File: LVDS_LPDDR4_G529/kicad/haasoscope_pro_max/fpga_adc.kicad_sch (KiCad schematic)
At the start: 0 parts

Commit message: Aligned schematics, sort of
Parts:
- added IC1: ADC12DL500ACF_Aligned, ADC12DL:BGA256C100P16X16_1700X1700X331, symbol Aligned_Peripheral_Symbols:ADC12DL500ACF_Aligned
- added U3: Ti90G529_Functions, G529:BGA-529_23x23_19.0x19.0mm, symbol Ti90G529_Functions:Ti90G529_Functions

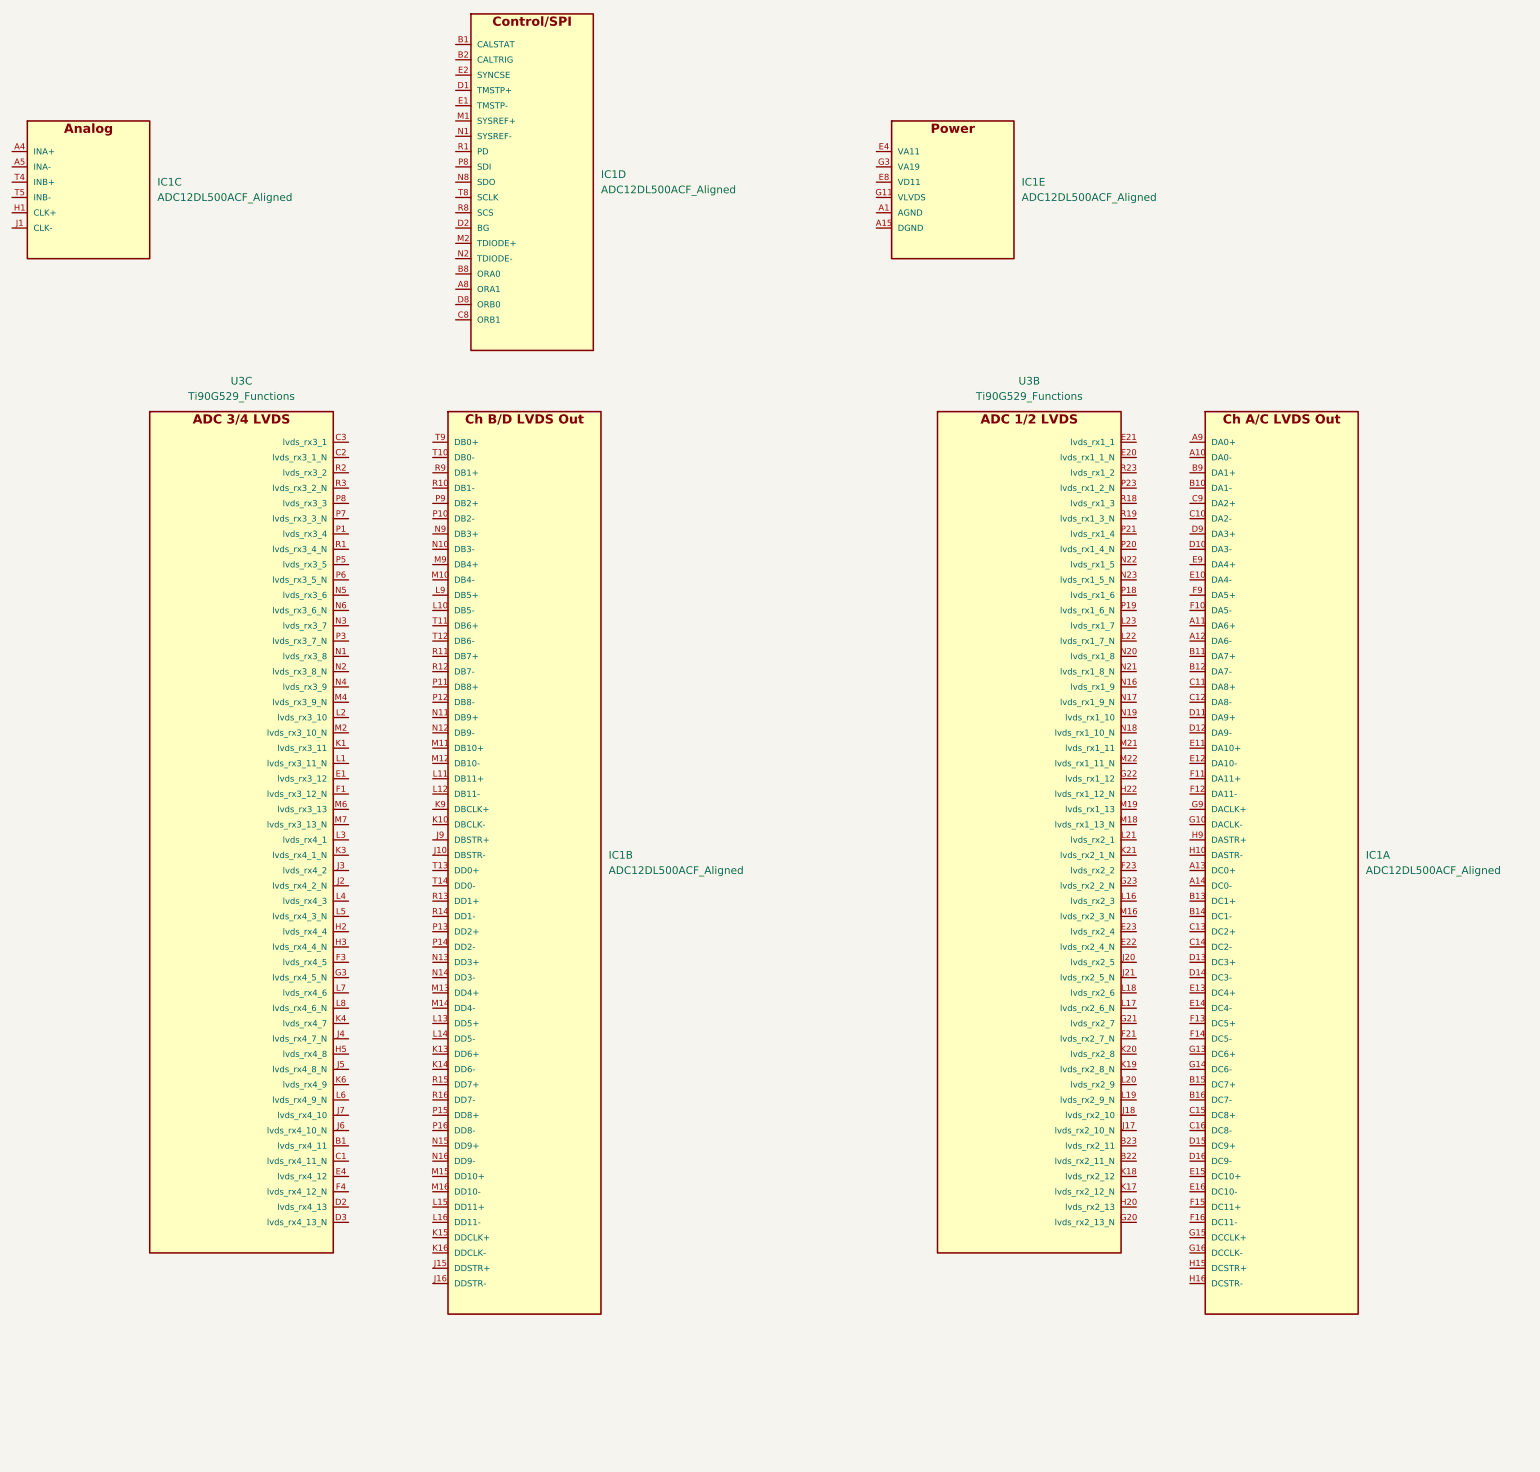
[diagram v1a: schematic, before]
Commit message: Aligned schematics, sort of
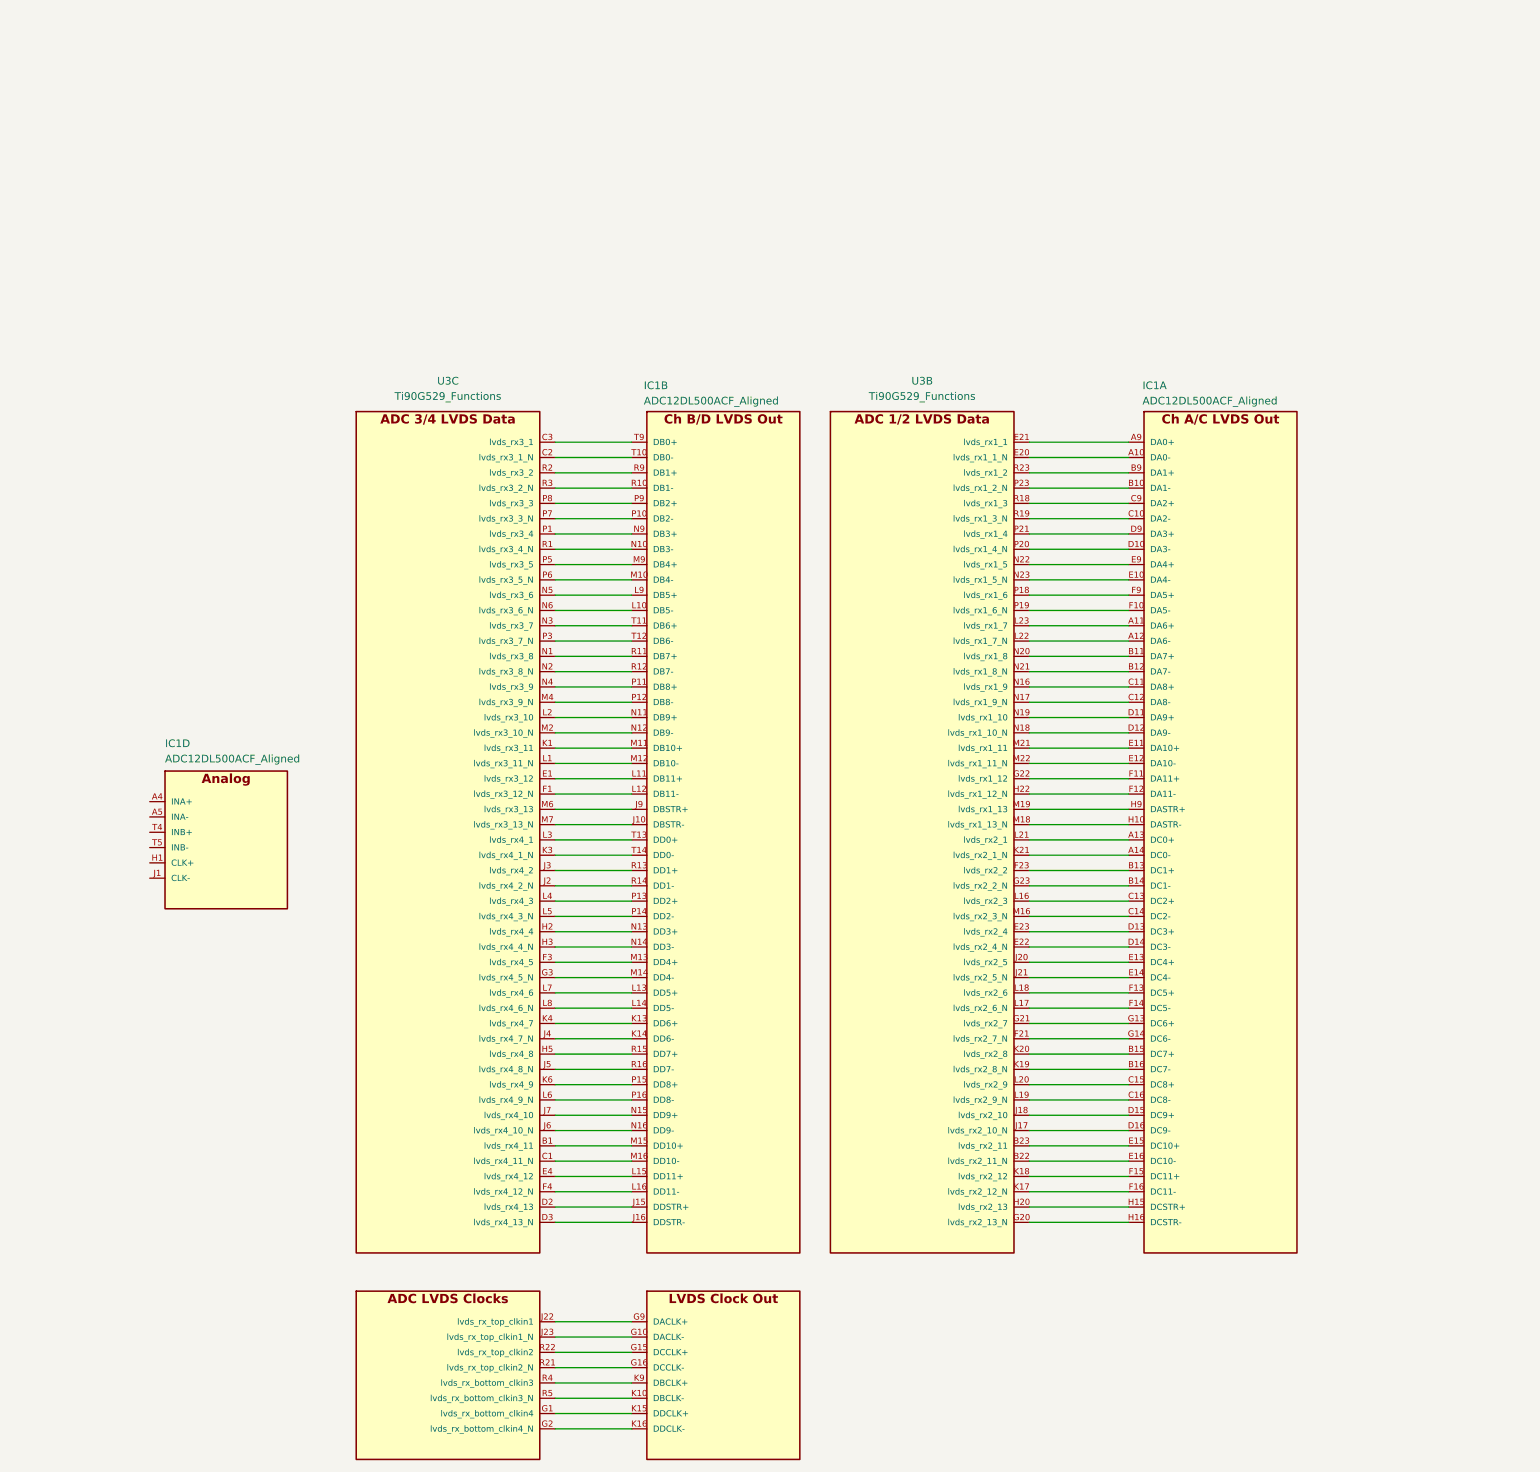
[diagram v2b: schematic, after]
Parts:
- removed unit 5 of IC1
- added unit 4 of U3
- IC1: footprint ADC12DL:BGA256C100P16X16_1700X1700X331 -> BGA256C100P16X16_1700X1700X331
- U3: footprint G529:BGA-529_23x23_19.0x19.0mm -> haasoscope_pro_adc_fpga_board:BGA-529_23x23_19.0x19.0mm
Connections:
- net at U3.B1 (lvds_rx4_11): now also IC1.M15 (DD10+)
- net at U3.C1 (lvds_rx4_11_N): now also IC1.M16 (DD10-)
- net at U3.C2 (lvds_rx3_1_N): now also IC1.T10 (DB0-)
- net at U3.C3 (lvds_rx3_1): now also IC1.T9 (DB0+)
- net at U3.D2 (lvds_rx4_13): now also IC1.J15 (DDSTR+)
- net at U3.D3 (lvds_rx4_13_N): now also IC1.J16 (DDSTR-)
- net at U3.E1 (lvds_rx3_12): now also IC1.L11 (DB11+)
- net at U3.E4 (lvds_rx4_12): now also IC1.L15 (DD11+)
- net at U3.F1 (lvds_rx3_12_N): now also IC1.L12 (DB11-)
- net at U3.F3 (lvds_rx4_5): now also IC1.M13 (DD4+)
- net at U3.F4 (lvds_rx4_12_N): now also IC1.L16 (DD11-)
- net at U3.G3 (lvds_rx4_5_N): now also IC1.M14 (DD4-)
- net at U3.H2 (lvds_rx4_4): now also IC1.N13 (DD3+)
- net at U3.H3 (lvds_rx4_4_N): now also IC1.N14 (DD3-)
- net at U3.H5 (lvds_rx4_8): now also IC1.R15 (DD7+)
- net at U3.J2 (lvds_rx4_2_N): now also IC1.R14 (DD1-)
- net at U3.J3 (lvds_rx4_2): now also IC1.R13 (DD1+)
- net at U3.J4 (lvds_rx4_7_N): now also IC1.K14 (DD6-)
- net at U3.J5 (lvds_rx4_8_N): now also IC1.R16 (DD7-)
- net at U3.J6 (lvds_rx4_10_N): now also IC1.N16 (DD9-)
- net at U3.J7 (lvds_rx4_10): now also IC1.N15 (DD9+)
- net at U3.K1 (lvds_rx3_11): now also IC1.M11 (DB10+)
- net at U3.K3 (lvds_rx4_1_N): now also IC1.T14 (DD0-)
- net at U3.K4 (lvds_rx4_7): now also IC1.K13 (DD6+)
- net at U3.K6 (lvds_rx4_9): now also IC1.P15 (DD8+)
- net at U3.L1 (lvds_rx3_11_N): now also IC1.M12 (DB10-)
- net at U3.L2 (lvds_rx3_10): now also IC1.N11 (DB9+)
- net at U3.L3 (lvds_rx4_1): now also IC1.T13 (DD0+)
- net at U3.L4 (lvds_rx4_3): now also IC1.P13 (DD2+)
- net at U3.L5 (lvds_rx4_3_N): now also IC1.P14 (DD2-)
- net at U3.L6 (lvds_rx4_9_N): now also IC1.P16 (DD8-)
- net at U3.L7 (lvds_rx4_6): now also IC1.L13 (DD5+)
- net at U3.L8 (lvds_rx4_6_N): now also IC1.L14 (DD5-)
- net at U3.M2 (lvds_rx3_10_N): now also IC1.N12 (DB9-)
- net at U3.M4 (lvds_rx3_9_N): now also IC1.P12 (DB8-)
- net at U3.M6 (lvds_rx3_13): now also IC1.J9 (DBSTR+)
- net at U3.M7 (lvds_rx3_13_N): now also IC1.J10 (DBSTR-)
- net at U3.N1 (lvds_rx3_8): now also IC1.R11 (DB7+)
- net at U3.N2 (lvds_rx3_8_N): now also IC1.R12 (DB7-)
- net at U3.N3 (lvds_rx3_7): now also IC1.T11 (DB6+)
- net at U3.N4 (lvds_rx3_9): now also IC1.P11 (DB8+)
- net at U3.N5 (lvds_rx3_6): now also IC1.L9 (DB5+)
- net at U3.N6 (lvds_rx3_6_N): now also IC1.L10 (DB5-)
- net at U3.P1 (lvds_rx3_4): now also IC1.N9 (DB3+)
- net at U3.P3 (lvds_rx3_7_N): now also IC1.T12 (DB6-)
- net at U3.P5 (lvds_rx3_5): now also IC1.M9 (DB4+)
- net at U3.P6 (lvds_rx3_5_N): now also IC1.M10 (DB4-)
- net at U3.P7 (lvds_rx3_3_N): now also IC1.P10 (DB2-)
- net at U3.P8 (lvds_rx3_3): now also IC1.P9 (DB2+)
- net at U3.R1 (lvds_rx3_4_N): now also IC1.N10 (DB3-)
- net at U3.R2 (lvds_rx3_2): now also IC1.R9 (DB1+)
- net at U3.R3 (lvds_rx3_2_N): now also IC1.R10 (DB1-)
- net at U3.B22 (lvds_rx2_11_N): now also IC1.E16 (DC10-)
- net at U3.B23 (lvds_rx2_11): now also IC1.E15 (DC10+)
- net at U3.E20 (lvds_rx1_1_N): now also IC1.A10 (DA0-)
- net at U3.E21 (lvds_rx1_1): now also IC1.A9 (DA0+)
- net at U3.E22 (lvds_rx2_4_N): now also IC1.D14 (DC3-)
- net at U3.E23 (lvds_rx2_4): now also IC1.D13 (DC3+)
- net at U3.F21 (lvds_rx2_7_N): now also IC1.G14 (DC6-)
- net at U3.F23 (lvds_rx2_2): now also IC1.B13 (DC1+)
- net at U3.G20 (lvds_rx2_13_N): now also IC1.H16 (DCSTR-)
- net at U3.G21 (lvds_rx2_7): now also IC1.G13 (DC6+)
- net at U3.G22 (lvds_rx1_12): now also IC1.F11 (DA11+)
- net at U3.G23 (lvds_rx2_2_N): now also IC1.B14 (DC1-)
- net at U3.H20 (lvds_rx2_13): now also IC1.H15 (DCSTR+)
- net at U3.H22 (lvds_rx1_12_N): now also IC1.F12 (DA11-)
- net at U3.J17 (lvds_rx2_10_N): now also IC1.D16 (DC9-)
- net at U3.J18 (lvds_rx2_10): now also IC1.D15 (DC9+)
- net at U3.J20 (lvds_rx2_5): now also IC1.E13 (DC4+)
- net at U3.J21 (lvds_rx2_5_N): now also IC1.E14 (DC4-)
- net at U3.K17 (lvds_rx2_12_N): now also IC1.F16 (DC11-)
- net at U3.K18 (lvds_rx2_12): now also IC1.F15 (DC11+)
- net at U3.K19 (lvds_rx2_8_N): now also IC1.B16 (DC7-)
- net at U3.K20 (lvds_rx2_8): now also IC1.B15 (DC7+)
- net at U3.K21 (lvds_rx2_1_N): now also IC1.A14 (DC0-)
- net at U3.L16 (lvds_rx2_3): now also IC1.C13 (DC2+)
- net at U3.L17 (lvds_rx2_6_N): now also IC1.F14 (DC5-)
- net at U3.L18 (lvds_rx2_6): now also IC1.F13 (DC5+)
- net at U3.L19 (lvds_rx2_9_N): now also IC1.C16 (DC8-)
- net at U3.L20 (lvds_rx2_9): now also IC1.C15 (DC8+)
- net at U3.L21 (lvds_rx2_1): now also IC1.A13 (DC0+)
- net at U3.L22 (lvds_rx1_7_N): now also IC1.A12 (DA6-)
- net at U3.L23 (lvds_rx1_7): now also IC1.A11 (DA6+)
- net at U3.M16 (lvds_rx2_3_N): now also IC1.C14 (DC2-)
- net at U3.M18 (lvds_rx1_13_N): now also IC1.H10 (DASTR-)
- net at U3.M19 (lvds_rx1_13): now also IC1.H9 (DASTR+)
- net at U3.M21 (lvds_rx1_11): now also IC1.E11 (DA10+)
- net at U3.M22 (lvds_rx1_11_N): now also IC1.E12 (DA10-)
- net at U3.N16 (lvds_rx1_9): now also IC1.C11 (DA8+)
- net at U3.N17 (lvds_rx1_9_N): now also IC1.C12 (DA8-)
- net at U3.N18 (lvds_rx1_10_N): now also IC1.D12 (DA9-)
- net at U3.N19 (lvds_rx1_10): now also IC1.D11 (DA9+)
- net at U3.N20 (lvds_rx1_8): now also IC1.B11 (DA7+)
- net at U3.N21 (lvds_rx1_8_N): now also IC1.B12 (DA7-)
- net at U3.N22 (lvds_rx1_5): now also IC1.E9 (DA4+)
- net at U3.N23 (lvds_rx1_5_N): now also IC1.E10 (DA4-)
- net at U3.P18 (lvds_rx1_6): now also IC1.F9 (DA5+)
- net at U3.P19 (lvds_rx1_6_N): now also IC1.F10 (DA5-)
- net at U3.P20 (lvds_rx1_4_N): now also IC1.D10 (DA3-)
- net at U3.P21 (lvds_rx1_4): now also IC1.D9 (DA3+)
- net at U3.P23 (lvds_rx1_2_N): now also IC1.B10 (DA1-)
- net at U3.R18 (lvds_rx1_3): now also IC1.C9 (DA2+)
- net at U3.R19 (lvds_rx1_3_N): now also IC1.C10 (DA2-)
- net at U3.R23 (lvds_rx1_2): now also IC1.B9 (DA1+)
- new net: IC1.K15 (DDCLK+), U3.G1 (lvds_rx_bottom_clkin4)
- new net: IC1.K16 (DDCLK-), U3.G2 (lvds_rx_bottom_clkin4_N)
- new net: IC1.G9 (DACLK+), U3.J22 (lvds_rx_top_clkin1)
- new net: IC1.G10 (DACLK-), U3.J23 (lvds_rx_top_clkin1_N)
- new net: IC1.G16 (DCCLK-), U3.R21 (lvds_rx_top_clkin2_N)
- new net: IC1.G15 (DCCLK+), U3.R22 (lvds_rx_top_clkin2)
- new net: IC1.K9 (DBCLK+), U3.R4 (lvds_rx_bottom_clkin3)
- new net: IC1.K10 (DBCLK-), U3.R5 (lvds_rx_bottom_clkin3_N)
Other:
- moved on the sheet: U3B, U3C
